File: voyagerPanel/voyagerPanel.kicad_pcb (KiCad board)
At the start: 2 copper layers, 70 x 50 mm, 44 parts, among them J1 USB_C_Receptacle_USB2.0_16P, J2 Battery Pin, J3 E-ink, J4 BME280_MODULE, SW1 SW_Push_45deg, SW2 SW_Push_45deg, SW3 SW_Push_45deg, SW4 SW_Push_45deg, U1 ESP32-S3-MINI-1, U2 MCP1700x-330xxMB, U4 TP4056-42-ESOP8

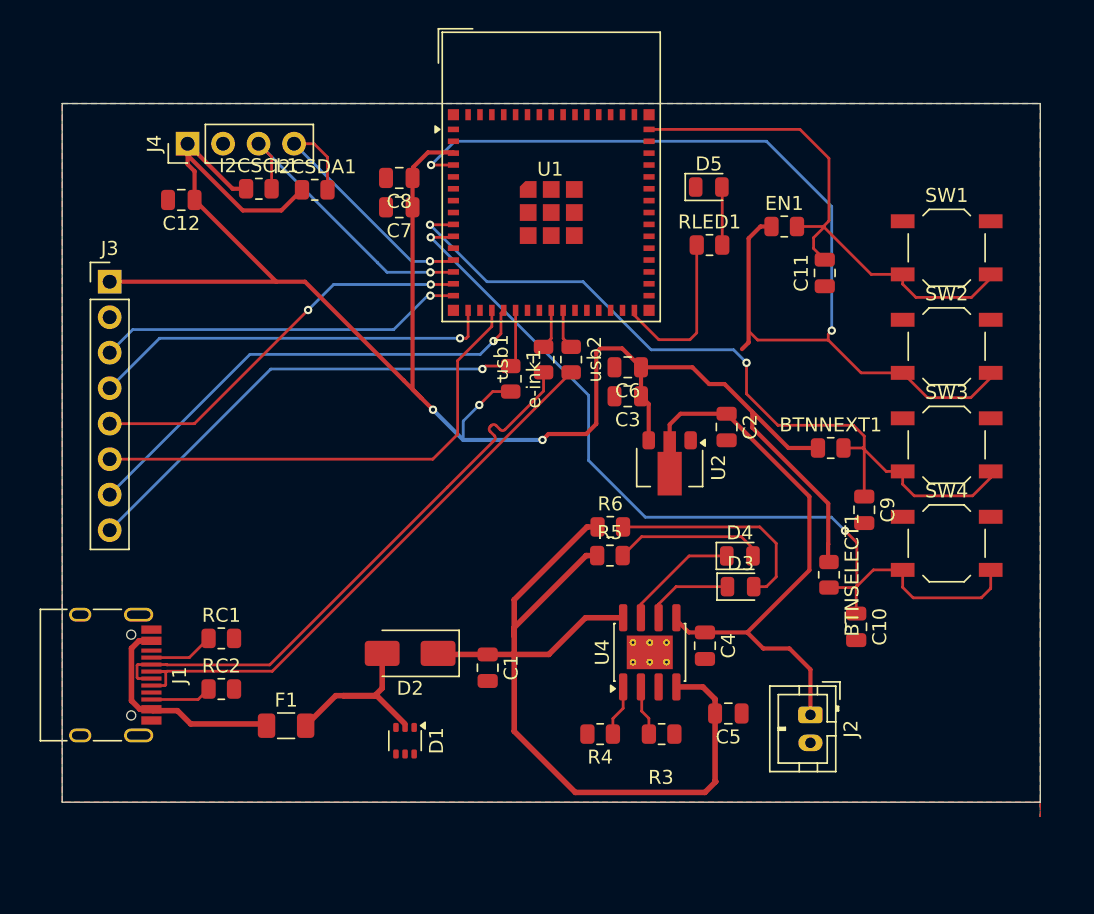
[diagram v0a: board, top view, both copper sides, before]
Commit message: finished PCB
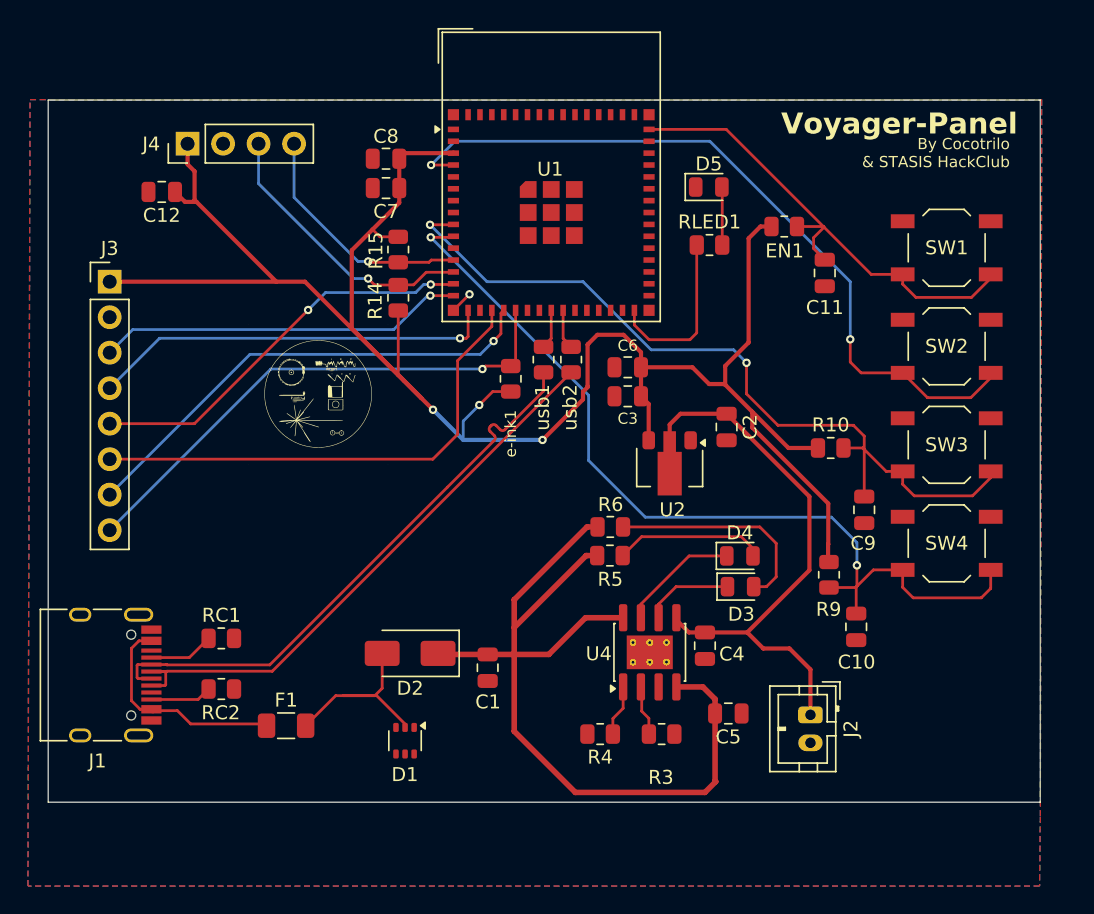
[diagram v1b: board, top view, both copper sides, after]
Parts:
- added G***: LOGO, LOGO, F.Cu at (42.2, 81.5)
- moved R14 12.7 mm to (48.0, 74.5), turned to 90 degrees
- moved R15 7.35 mm to (48.0, 71.1), turned to -90 degrees
- moved C7 1.67 mm to (47.1, 66.7)
- moved C8 1.67 mm to (47.1, 64.6)
- moved C12 1.51 mm to (31.0, 67.0)
- renumbered BTNNEXT1 to R10, I2CSCL1 to R14, I2CSDA1 to R15, BTNSELECT1 to R9
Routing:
- net PROG_IO0: track 72.9 -> 54.3 mm
- net +3V3: track 137.5 -> 147.6 mm
- net PROG_EN: track 39.0 -> 35.6 mm
- net I2C_SDA: track 20.1 -> 17.4 mm
- net GND: track 0.00 -> 1.63 mm, vias 0 -> 1
- net I2C_SCL: track 22.1 -> 20.9 mm
- net +5V: track 66.2 -> 65.6 mm
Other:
- board size 70 x 50 mm -> 71 x 50.3 mm
- board text added: "By Cocotrilo & STASIS HackClub"
- board text added: "VP"
- board text added: "Voyager-Panel"
